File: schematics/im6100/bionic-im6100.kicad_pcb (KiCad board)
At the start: 2 copper layers, 25.4 x 68.6 mm, 8 parts, among them J1 Bionic-P135, J2 Bionic-P245, U1 IM6100, U2 11AA010-I/TT

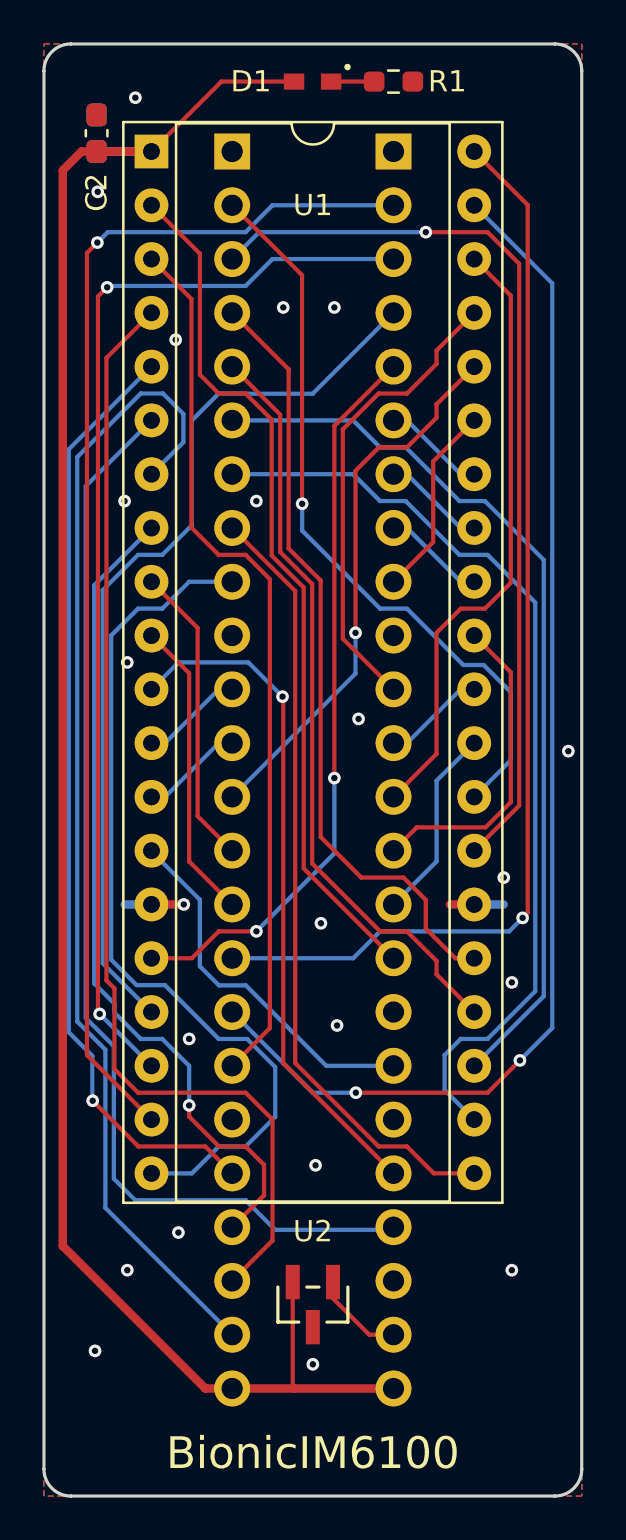
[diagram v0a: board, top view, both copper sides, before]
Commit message: [IM6100] Cleanup schematics
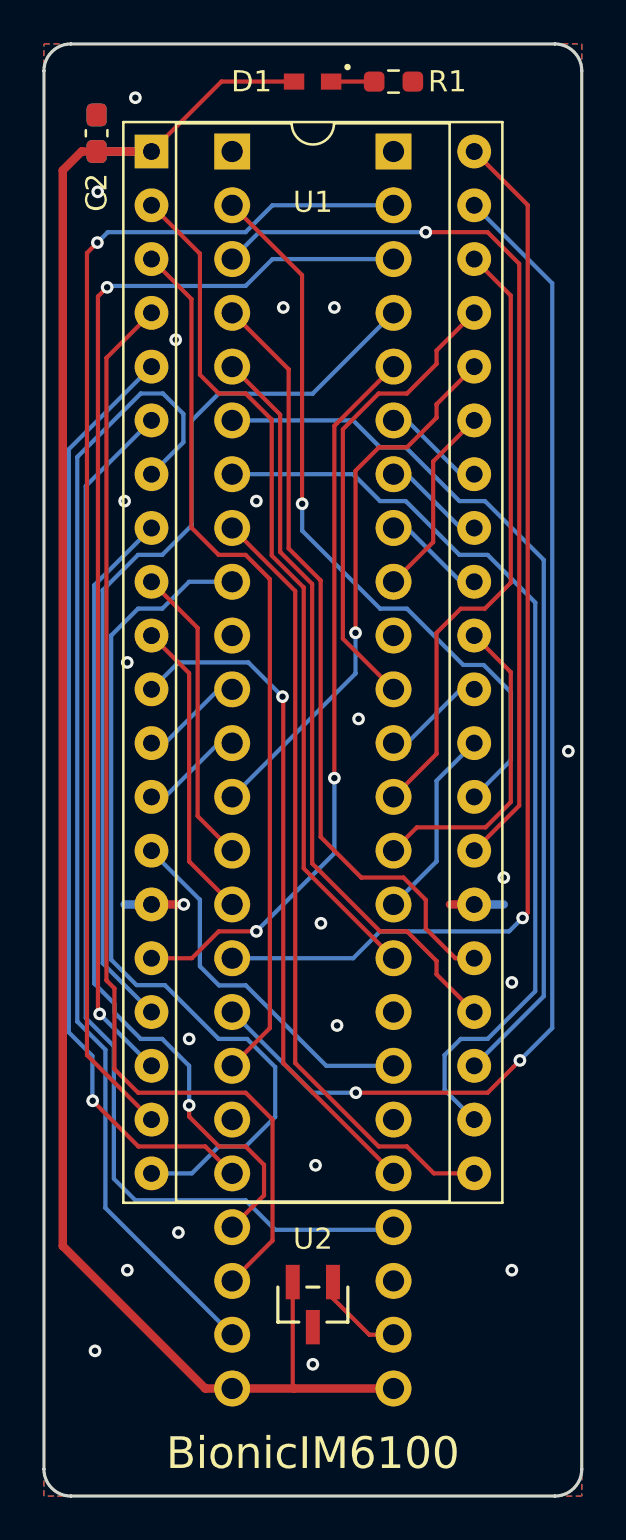
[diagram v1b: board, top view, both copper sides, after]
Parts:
- D1: footprint 0-LocalLibrary:LED_CSL1901UW1_ROM-M -> rhom:LED_CSL1901UW1_ROM-M
- J1: footprint 0-LocalLibrary:Bionic-P135_Vertical -> bionic:Bionic-P135_Vertical
- J2: footprint 0-LocalLibrary:Bionic-P245_Vertical -> bionic:Bionic-P245_Vertical
- U1: footprint 0-LocalLibrary:DIP-40_W15.24mm_Socket -> bionic:DIP-40_W15.24mm_Socket
- U2: footprint 0-LocalLibrary:SOT-23_MC_MCH-M -> microchip:SOT-23_MC_MCH-M
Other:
- rule pad_to_mask_clearance: 0.051 -> 0
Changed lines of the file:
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@@
 			(dielectric_constraints no)
 		)
-		(pad_to_mask_clearance 0.051)
-		(solder_mask_min_width 0.25)
+		(pad_to_mask_clearance 0)
 		(allow_soldermask_bridges_in_footprints no)
 		(aux_axis_origin 101 70)
@@
 	(net 46 "/P33")
 	(net 47 "unconnected-(J2-P46-Pad32)")
-	(footprint "0-LocalLibrary:SOT-23_MC_MCH-M"
+	(footprint "microchip:SOT-23_MC_MCH-M"
 		(locked yes)
 		(layer "F.Cu")
@@
 		(descr "Microchip 11AAxxx-I/TT UNI/O 1Kbit Serial EEPROM")
 		(property "Reference" "U2"
-			(at 0 3.4544 0)
+			(at 0 3.0988 0)
 			(unlocked yes)
 			(layer "F.SilkS")
@@
 			)
 		)
-		(property "Footprint" "0-LocalLibrary:SOT-23_MC_MCH-M"
+		(property "Footprint" "microchip:SOT-23_MC_MCH-M"
 			(at 0 0 180)
 			(layer "F.Fab")
@@
 			)
 		)
-		(property "Description" ""
+		(property "Description" "UNI/O Serial EEPROM (1Kbit)"
 			(at 0 0 180)
 			(layer "F.Fab")
@@
 			(pintype "power_in")
 		)
-		(model "${KIPRJMOD}/0-LocalLibrary/SOT-23_MC_MCH.step"
+		(model "${KIPRJMOD}/microchip.pretty/SOT-23_MC_MCH.step"
 			(offset
 				(xyz 0 0 0)
@@
 		)
 	)
-	(footprint "0-LocalLibrary:LED_CSL1901UW1_ROM-M"
+	(footprint "rhom:LED_CSL1901UW1_ROM-M"
 		(layer "F.Cu")
 		(at 113.6873 71.778 180)
@@
 		(tags "CSL1901UW1 ")
 		(property "Reference" "D1"
-			(at 2.9083 0 0)
+			(at 2.8829 0 0)
 			(unlocked yes)
 			(layer "F.SilkS")
@@
 			)
 		)
-		(property "Footprint" "0-LocalLibrary:LED_CSL1901UW1_ROM-M"
-			(at 0 0 360)
+		(property "Footprint" "rhom:LED_CSL1901UW1_ROM-M"
+			(at 0 0 180)
 			(layer "F.Fab")
 			(hide yes)
@@
 		)
 		(property "Datasheet" "https://fscdn.rohm.com/en/products/databook/datasheet/opto/led/chip_mono/csl1901uw1-e.pdf"
-			(at 0 0 360)
+			(at 0 0 180)
 			(layer "F.Fab")
 			(hide yes)
@@
 		)
 		(property "Description" "Red LED (Low Current Emission, SMD)"
-			(at 0 0 360)
+			(at 0 0 180)
 			(layer "F.Fab")
 			(hide yes)
@@
 			)
 		)
-		(model "${KIPRJMOD}/0-LocalLibrary/LED_CSL1901UW1_ROM.step"
+		(model "${KIPRJMOD}/rhom.pretty/LED_CSL1901UW1_ROM.step"
 			(offset
 				(xyz 0 0 0)
@@
 		)
 	)
-	(footprint "0-LocalLibrary:DIP-40_W15.24mm_Socket"
+	(footprint "bionic:DIP-40_W15.24mm_Socket"
 		(locked yes)
 		(layer "F.Cu")
@@
 		(tags "THT DIP DIL PDIP 2.54mm 15.24mm 600mil Socket")
 		(property "Reference" "U1"
-			(at 7.62 2.54 0)
+			(at 7.62 2.3876 0)
 			(layer "F.SilkS")
 			(effects
@@
 			)
 		)
-		(property "Footprint" "0-LocalLibrary:DIP-40_W15.24mm_Socket"
+		(property "Footprint" "bionic:DIP-40_W15.24mm_Socket"
 			(at 0 0 0)
 			(layer "F.Fab")
@@
 		)
 	)
-	(footprint "0-LocalLibrary:Bionic-P245_Vertical"
+	(footprint "bionic:Bionic-P245_Vertical"
 		(locked yes)
 		(layer "B.Cu")
@@
 			)
 		)
-		(property "Footprint" "0-LocalLibrary:Bionic-P245_Vertical"
-			(at 0 0 180)
-			(layer "F.Fab")
+		(property "Footprint" "bionic:Bionic-P245_Vertical"
+			(at 0 0 0)
+			(layer "B.Fab")
 			(hide yes)
 			(effects
@@
 					(thickness 0.15)
 				)
+				(justify mirror)
 			)
 		)
 		(property "Datasheet" ""
-			(at 0 0 180)
-			(layer "F.Fab")
+			(at 0 0 0)
+			(layer "B.Fab")
 			(hide yes)
 			(effects
@@
 					(thickness 0.15)
 				)
-			)
-		)
-		(property "Description" ""
-			(at 0 0 180)
-			(layer "F.Fab")
+				(justify mirror)
+			)
+		)
+		(property "Description" "Generic connector, single row, 01x24, script generated (kicad-library-utils/schlib/autogen/connector/)"
+			(at 0 0 0)
+			(layer "B.Fab")
 			(hide yes)
 			(effects
@@
 					(thickness 0.15)
 				)
+				(justify mirror)
 			)
 		)
@@
 		)
 	)
-	(footprint "0-LocalLibrary:Bionic-P135_Vertical"
+	(footprint "bionic:Bionic-P135_Vertical"
 		(locked yes)
 		(layer "B.Cu")
@@
 			)
 		)
-		(property "Footprint" "0-LocalLibrary:Bionic-P135_Vertical"
-			(at 0 0 180)
-			(layer "F.Fab")
+		(property "Footprint" "bionic:Bionic-P135_Vertical"
+			(at 0 0 0)
+			(layer "B.Fab")
 			(hide yes)
 			(effects
@@
 					(thickness 0.15)
 				)
+				(justify mirror)
 			)
 		)
 		(property "Datasheet" ""
-			(at 0 0 180)
-			(layer "F.Fab")
+			(at 0 0 0)
+			(layer "B.Fab")
 			(hide yes)
 			(effects
@@
 					(thickness 0.15)
 				)
-			)
-		)
-		(property "Description" ""
-			(at 0 0 180)
-			(layer "F.Fab")
+				(justify mirror)
+			)
+		)
+		(property "Description" "Generic connector, single row, 01x24, script generated (kicad-library-utils/schlib/autogen/connector/)"
+			(at 0 0 0)
+			(layer "B.Fab")
 			(hide yes)
 			(effects
@@
 					(thickness 0.15)
 				)
-			)
-		)
+				(justify mirror)
+			)
+		)
